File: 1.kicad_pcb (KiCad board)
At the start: 2 copper layers, 55.9 x 35.6 mm, 24 parts, among them J1 Screw_Terminal_01x03, J2 Screw_Terminal_01x01, J3 Screw_Terminal_01x01, U1 LTC2990, U2 LTC2990, U3 LTC2990

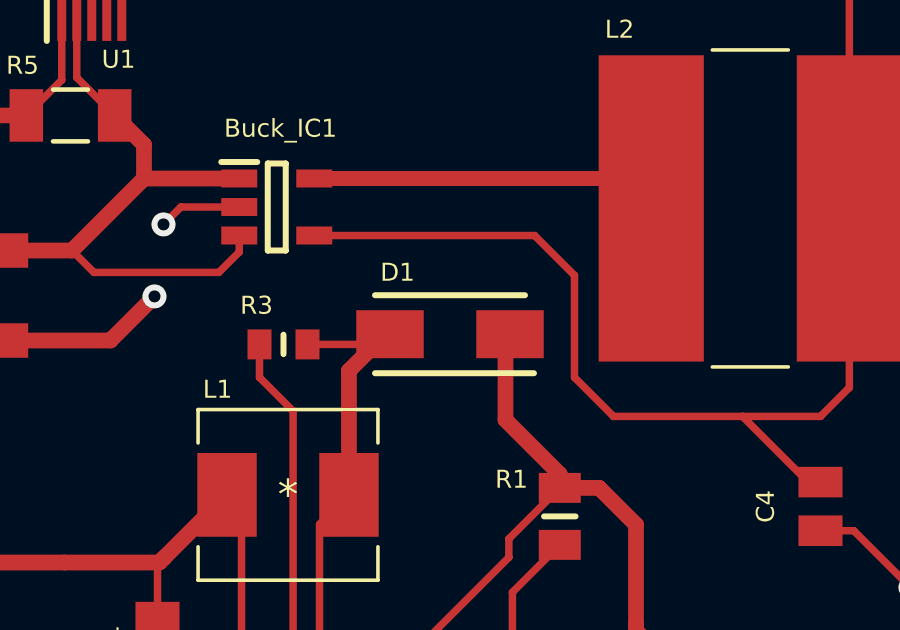
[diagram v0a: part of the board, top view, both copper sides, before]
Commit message: FInal...I guess
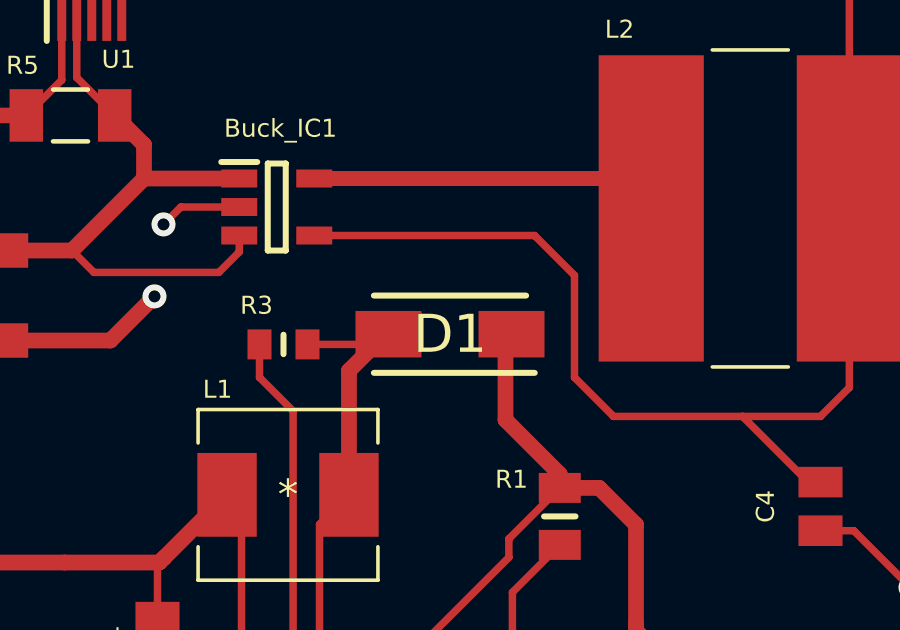
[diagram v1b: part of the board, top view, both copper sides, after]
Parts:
- D1: footprint Schottky dd:DIOM5026X220N -> Schottky DD with stock:DIOM5126X265N
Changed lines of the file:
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@@
       (sketchpadsonfab false)
       (subtractmaskfromsilk false)
-      (outputformat 4)
+      (outputformat 1)
       (mirror false)
       (drillshape 0)
       (scaleselection 1)
-      (outputdirectory "/home/arch1/Desktop/")
+      (outputdirectory "/mnt/DAA829C1A8299CCF/EEE/S7/PROJ/voltage-regulator-module/Gerbers/")
     )
   )
@@
     )
   )
-  (footprint "Schottky dd:DIOM5026X220N" (layer "F.Cu")
+  (footprint "Schottky DD with stock:DIOM5126X265N" (layer "F.Cu")
     (at 152.55 86.36 180)
-    (descr "PMDS_SOD106")
-    (tags "Schottky Diode")
-    (property "Sheetfile" "1.kicad_sch")
-    (property "Sheetname" "")
-    (attr smd)
-    (fp_text reference "D1" (at 1.75 2.06 180) (layer "F.SilkS")
-      (effects (font (size 0.6 0.6) (thickness 0.15)))
+    (descr "SMA")
+    (tags "Diode")
+    (property "Sheetfile" "1.kicad_sch")
+    (property "Sheetname" "")
+    (attr smd)
+    (fp_text reference "D1" (at 0 0 180) (layer "F.SilkS")
+      (effects (font (size 1.27 1.27) (thickness 0.254)))
     )
     (fp_text value "D_Schottky" (at 0 0 180) (layer "F.SilkS") hide
@@
       (effects (font (size 1.27 1.27) (thickness 0.254)))
     )
-    (fp_line (start 2.5 -1.3) (end -2.8 -1.3) (layer "F.SilkS") (width 0.2))
-    (fp_line (start -2.5 1.3) (end 2.5 1.3) (layer "F.SilkS") (width 0.2))
-    (fp_line (start -3.375 1.65) (end -3.375 -1.65) (layer "F.CrtYd") (width 0.05))
-    (fp_line (start -3.375 -1.65) (end 3.375 -1.65) (layer "F.CrtYd") (width 0.05))
-    (fp_line (start 3.375 -1.65) (end 3.375 1.65) (layer "F.CrtYd") (width 0.05))
-    (fp_line (start 3.375 1.65) (end -3.375 1.65) (layer "F.CrtYd") (width 0.05))
-    (fp_line (start 2.5 1.3) (end -2.5 1.3) (layer "F.Fab") (width 0.1))
-    (fp_line (start -2.5 -0.5) (end -1.7 -1.3) (layer "F.Fab") (width 0.1))
-    (fp_line (start -2.5 1.3) (end -2.5 -1.3) (layer "F.Fab") (width 0.1))
-    (fp_line (start 2.5 -1.3) (end 2.5 1.3) (layer "F.Fab") (width 0.1))
-    (fp_line (start -2.5 -1.3) (end 2.5 -1.3) (layer "F.Fab") (width 0.1))
-    (pad "1" smd rect (at -2 0 270) (size 1.6 2.25) (layers "F.Cu" "F.Paste" "F.Mask")
+    (fp_line (start -2.538 1.288) (end 2.538 1.288) (layer "F.SilkS") (width 0.2))
+    (fp_line (start 2.538 -1.288) (end -2.825 -1.288) (layer "F.SilkS") (width 0.2))
+    (fp_line (start -3.4 1.7) (end -3.4 -1.7) (layer "F.CrtYd") (width 0.05))
+    (fp_line (start 3.4 1.7) (end -3.4 1.7) (layer "F.CrtYd") (width 0.05))
+    (fp_line (start -3.4 -1.7) (end 3.4 -1.7) (layer "F.CrtYd") (width 0.05))
+    (fp_line (start 3.4 -1.7) (end 3.4 1.7) (layer "F.CrtYd") (width 0.05))
+    (fp_line (start 2.538 1.288) (end -2.538 1.288) (layer "F.Fab") (width 0.1))
+    (fp_line (start -2.538 -0.512) (end -1.762 -1.288) (layer "F.Fab") (width 0.1))
+    (fp_line (start -2.538 1.288) (end -2.538 -1.288) (layer "F.Fab") (width 0.1))
+    (fp_line (start 2.538 -1.288) (end 2.538 1.288) (layer "F.Fab") (width 0.1))
+    (fp_line (start -2.538 -1.288) (end 2.538 -1.288) (layer "F.Fab") (width 0.1))
+    (pad "1" smd rect (at -2.05 0 270) (size 1.55 2.2) (layers "F.Cu" "F.Paste" "F.Mask")
       (net 8 "Net-(Boost_IC1-Pad5)") (pinfunction "K") (pintype "passive"))
-    (pad "2" smd rect (at 2 0 270) (size 1.6 2.25) (layers "F.Cu" "F.Paste" "F.Mask")
+    (pad "2" smd rect (at 2.05 0 270) (size 1.55 2.2) (layers "F.Cu" "F.Paste" "F.Mask")
       (net 5 "Net-(Boost_IC1-Pad6)") (pinfunction "A") (pintype "passive"))
-    (model "RBR3L40ADDTE25.stp"
-      (offset (xyz 0 0 0))
-      (scale (xyz 1 1 1))
-      (rotate (xyz 0 0 0))
-    )
-    (model "/mnt/DAA829C1A8299CCF/EEE/S7/PROJ/COMPS/Schottky/LIB_RBR3L40ADDTE25/RBR3L40ADDTE25/3D/RBR3L40ADDTE25.stp"
-      (offset (xyz 0 0 0))
-      (scale (xyz 1 1 1))
-      (rotate (xyz 0 0 0))
+    (model "STPS2150A.stp" hide
+      (offset (xyz 0 0 0.23))
+      (scale (xyz 1 1 1))
+      (rotate (xyz 0 0 -180))
+    )
+    (model "/mnt/DAA829C1A8299CCF/EEE/S7/PROJ/COMPS/Schottky/LIB_STPS2150A stock ond/STPS2150A/3D/STPS2150A.stp"
+      (offset (xyz 0 0 1.1))
+      (scale (xyz 1 1 1))
+      (rotate (xyz 0 0 0))
